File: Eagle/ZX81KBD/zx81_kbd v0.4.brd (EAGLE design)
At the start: 100.5 x 82.5 mm, 119 parts, among them IC1 REG1117, IC3 PCF8574P

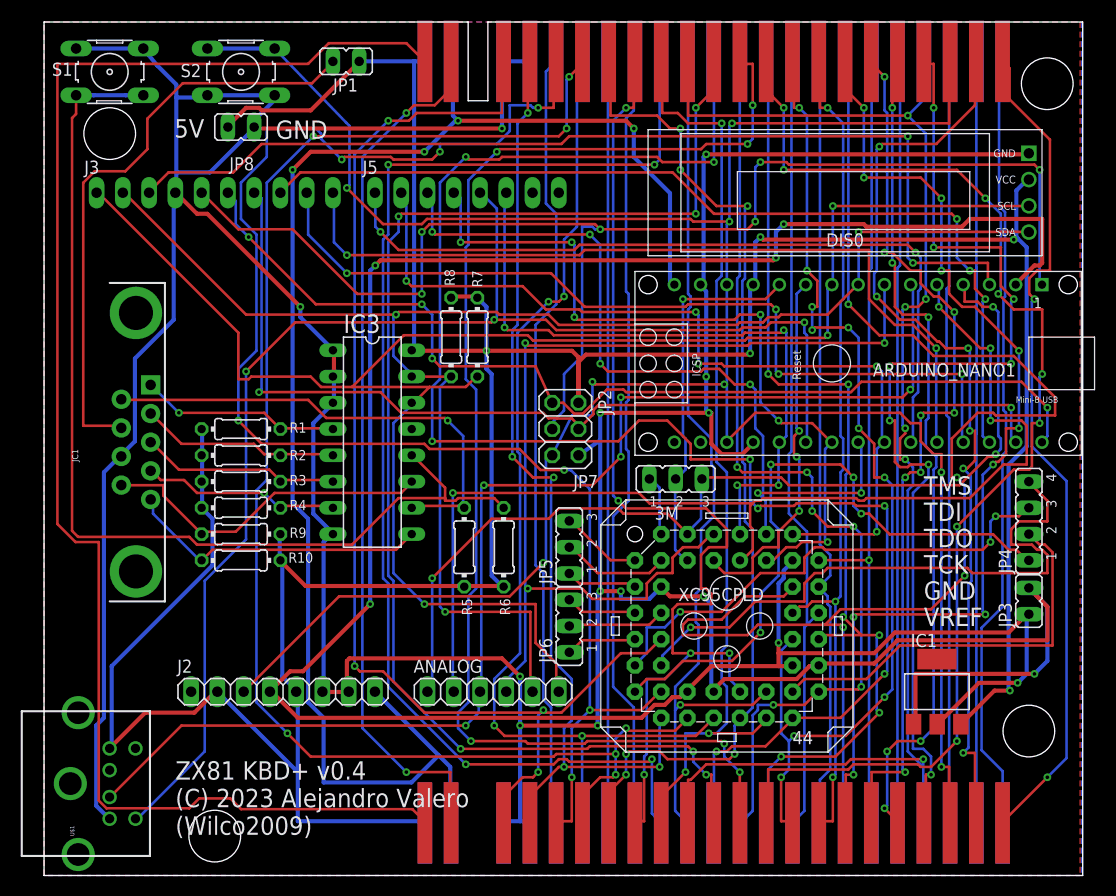
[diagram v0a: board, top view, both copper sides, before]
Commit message: update
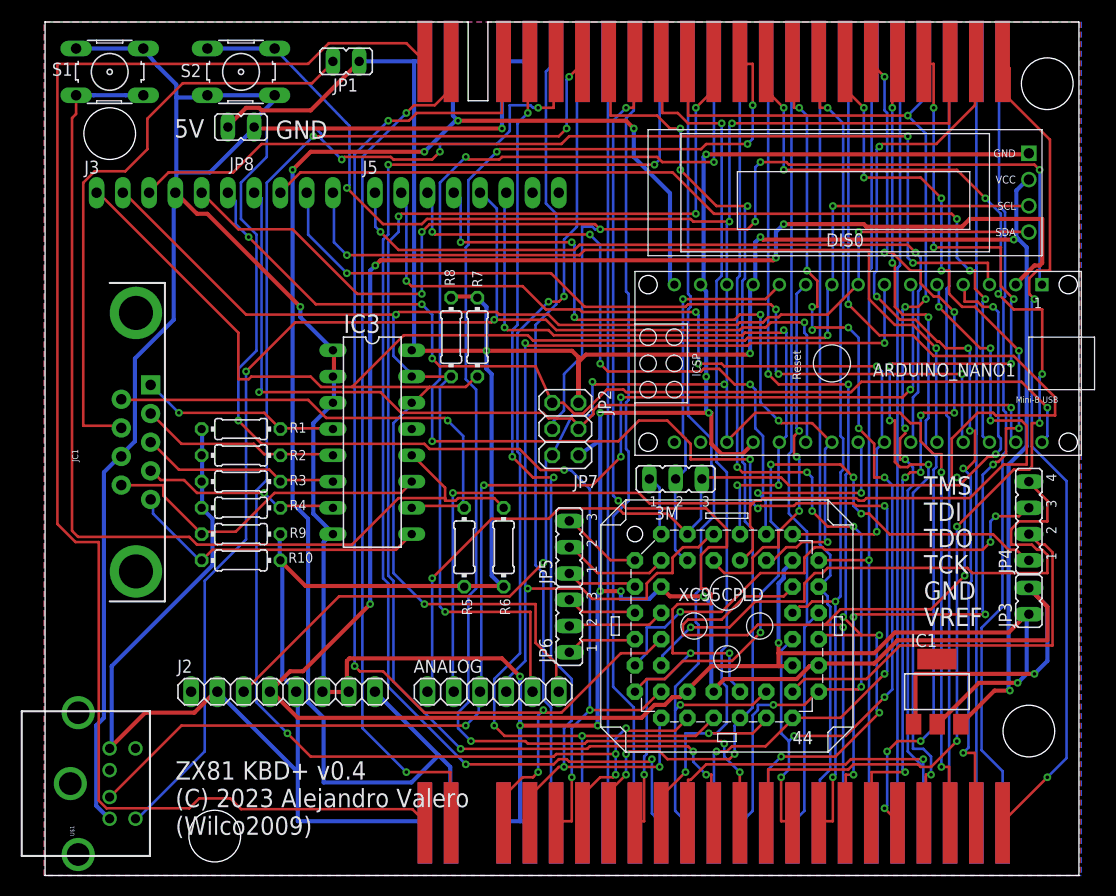
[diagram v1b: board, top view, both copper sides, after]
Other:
- board size 100.5 x 82.5 mm -> 100 x 82.5 mm
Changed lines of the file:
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@@
 <board>
 <plain>
-<wire x1="66.167" y1="0" x2="66.167" y2="82.55" width="0" layer="20"/>
-<wire x1="-34.29" y1="0" x2="-34.29" y2="82.55" width="0" layer="20"/>
-<wire x1="-34.29" y1="82.55" x2="6.731" y2="82.55" width="0" layer="20"/>
-<wire x1="8.636" y1="82.55" x2="66.167" y2="82.55" width="0" layer="20"/>
-<wire x1="66.167" y1="0" x2="-34.29" y2="0" width="0" layer="20"/>
+<wire x1="65.8" y1="0" x2="65.8" y2="82.55" width="0" layer="20"/>
+<wire x1="-34.19" y1="0" x2="-34.19" y2="82.55" width="0" layer="20"/>
+<wire x1="-34.19" y1="82.55" x2="6.731" y2="82.55" width="0" layer="20"/>
+<wire x1="8.636" y1="82.55" x2="65.8" y2="82.55" width="0" layer="20"/>
+<wire x1="65.8" y1="0" x2="-34.19" y2="0" width="0" layer="20"/>
 <wire x1="6.731" y1="82.55" x2="6.731" y2="74.93" width="0" layer="20"/>
 <wire x1="6.731" y1="74.93" x2="8.636" y2="74.93" width="0" layer="20"/>
